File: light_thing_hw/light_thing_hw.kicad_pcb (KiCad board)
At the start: 2 copper layers, 51 parts, among them J1 CONNECTORS, J2 Li-Ion Battery, J3 ADDR_LED_PANEL_1_CONNECTORS, J4 ADDR_LED_PANEL_2_CONNECTORS, Q1 MMBF170, SW1 ST_USER_BUTTON1, SW2 ST_RESET_BUTTON, U1 BC832-V1, U2 LSM6DS3, U3 MCP73833T-FCI_MF, U4 LMR62421XMF, U5 LP38511MRX-ADJ_NOPB, U5A1 STM32L452RETx

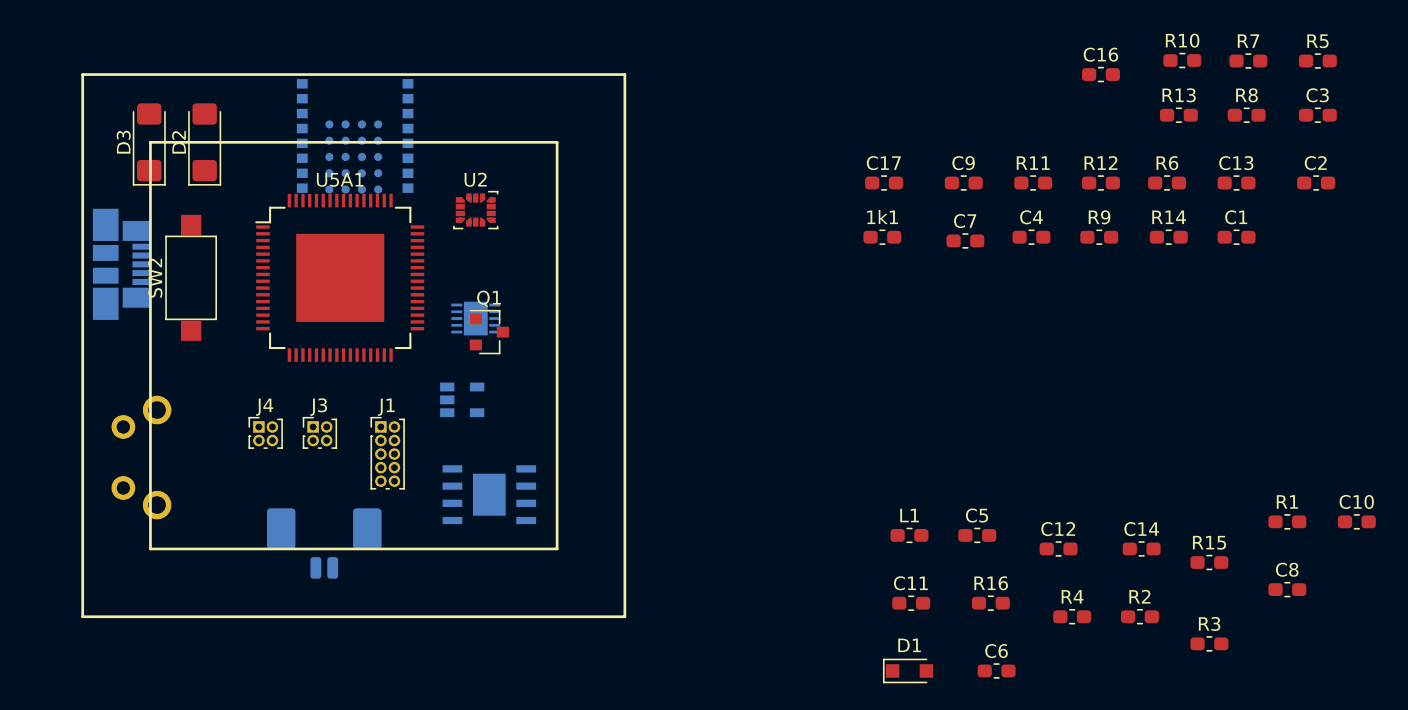
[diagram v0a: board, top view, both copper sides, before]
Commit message: hw updates
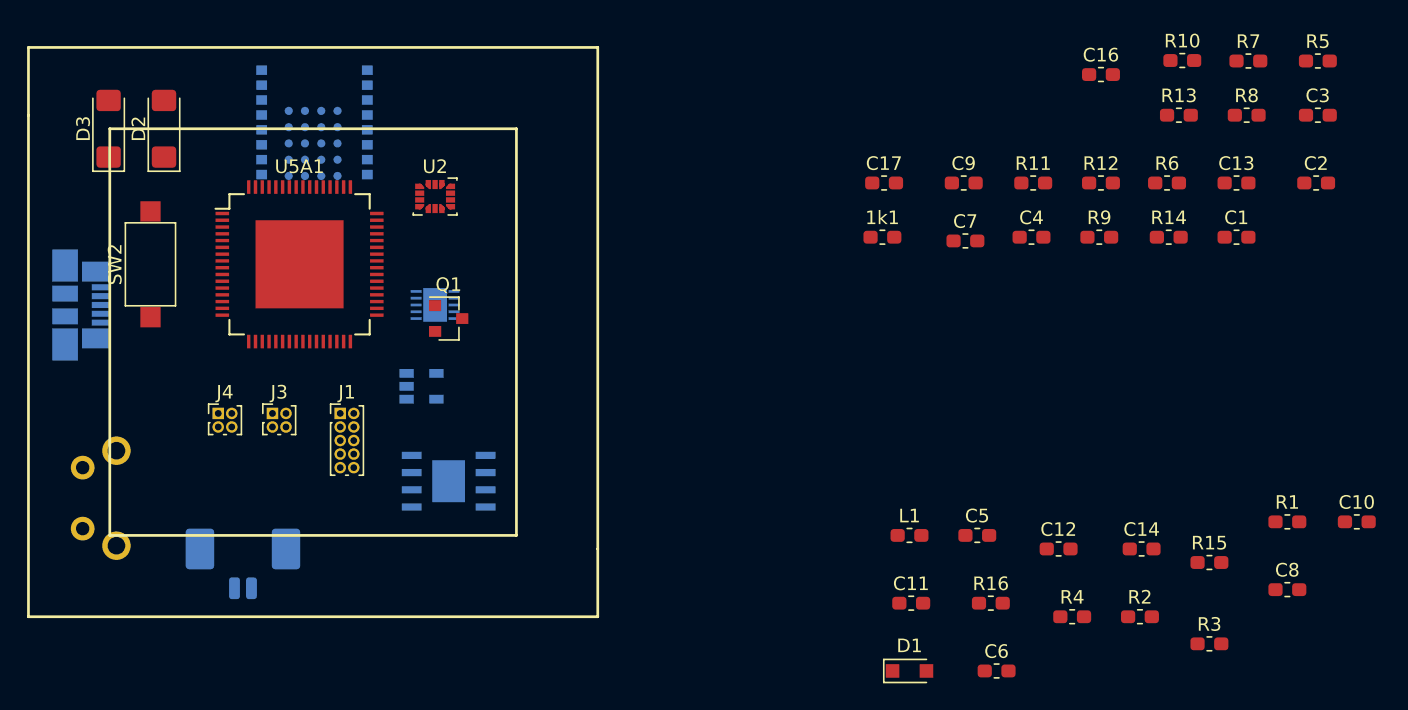
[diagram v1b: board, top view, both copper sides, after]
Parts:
- moved J2 6.18 mm to (166.8, 80.5)
- moved SW1 4.24 mm to (155.0, 74.0)
- moved USB_MICRO_CONN1 4.24 mm to (154.9, 62.0)
- moved D2 3.16 mm to (161.0, 49.0)
- moved D3 3.16 mm to (156.9, 49.0)
- moved J1 3.16 mm to (174.0, 70.0)
- moved J3 3.16 mm to (169.0, 70.0)
- moved J4 3.16 mm to (165.0, 70.0)
- moved Q1 3.16 mm to (182.0, 63.0)
- moved SW2 3.16 mm to (160.0, 59.0)
- moved U1 3.16 mm to (176.0, 53.0)
- moved U2 3.16 mm to (181.0, 54.0)
- moved U3 3.16 mm to (181.0, 62.0)
- moved U4 3.16 mm to (180.0, 68.0)
- moved U5 3.16 mm to (182.0, 75.0)
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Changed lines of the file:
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@@
   (general
     (thickness 1.6)
-    (drawings 11)
+    (drawings 12)
     (tracks 0)
     (zones 0)
@@
   )
   (module LED_SMD:LED_1806_4516Metric_Pad1.57x1.80mm_HandSolder (layer F.Cu)
-    (at 164 50 90)
+    (at 161 49 90)
     (descr "LED SMD 1806 (4516 Metric), square (rectangular) end terminal, IPC_7351 nominal, (Body size source: https://www.modelithics.com/models/Vendor/MuRata/BLM41P.pdf), generated with kicad-footprint-generator")
     (tags "LED handsolder")
@@
   )
   (module LED_SMD:LED_1806_4516Metric_Pad1.57x1.80mm_HandSolder (layer F.Cu)
-    (at 159.9125 50 90)
+    (at 156.9125 49 90)
     (descr "LED SMD 1806 (4516 Metric), square (rectangular) end terminal, IPC_7351 nominal, (Body size source: https://www.modelithics.com/models/Vendor/MuRata/BLM41P.pdf), generated with kicad-footprint-generator")
     (tags "LED handsolder")
@@
   )
   (module Connector_Molex:Molex_PicoBlade_53261-0271_1x02-1MP_P1.25mm_Horizontal (layer B.Cu)
-    (at 172.825 79)
+    (at 166.825 80.5)
     (descr "Molex PicoBlade series connector, 53261-0271 (http://www.molex.com/pdm_docs/sd/532610271_sd.pdf), generated with kicad-footprint-generator")
     (tags "connector Molex PicoBlade top entry")
@@
   )
   (module Connector_PinHeader_1.00mm:PinHeader_2x02_P1.00mm_Vertical (layer F.Cu)
-    (at 172 71)
+    (at 169 70)
     (descr "Through hole straight pin header, 2x02, 1.00mm pitch, double rows")
     (tags "Through hole pin header THT 2x02 1.00mm double row")
@@
   )
   (module Connector_PinHeader_1.00mm:PinHeader_2x02_P1.00mm_Vertical (layer F.Cu)
-    (at 168 71)
+    (at 165 70)
     (descr "Through hole straight pin header, 2x02, 1.00mm pitch, double rows")
     (tags "Through hole pin header THT 2x02 1.00mm double row")
@@
   )
   (module Package_TO_SOT_SMD:SOT-23 (layer F.Cu)
-    (at 185 64)
+    (at 182 63)
     (descr "SOT-23, Standard")
     (tags SOT-23)
@@
   )
   (module Button_Switch_THT:SW_Tactile_SPST_Angled_PTS645Vx39-2LFS (layer B.Cu)
-    (at 158 71 270)
+    (at 155 74 270)
     (descr "tactile switch SPST right angle, PTS645VL39-2 LFS")
     (tags "tactile switch SPST angled PTS645VL39-2 LFS C&K Button")
@@
   )
   (module Button_Switch_SMD:SW_SPST_CK_RS282G05A3 (layer F.Cu)
-    (at 163 60 90)
+    (at 160 59 90)
     (descr https://www.mouser.com/ds/2/60/RS-282G05A-SM_RT-1159762.pdf)
     (tags "SPST button tactile switch")
@@
   )
   (module Package_LGA:LGA-14_3x2.5mm_P0.5mm_LayoutBorder3x4y (layer F.Cu)
-    (at 184 55)
+    (at 181 54)
     (descr "LGA, 14 Pin (http://www.st.com/resource/en/datasheet/lsm6ds3.pdf), generated with kicad-footprint-generator ipc_lga_layoutBorder_generator.py")
     (tags "LGA LGA")
@@
   )
   (module footprints:MCP73833T-FCI&slash_MF (layer B.Cu)
-    (at 184 63)
+    (at 181 62)
     (fp_text reference U3 (at 0 3) (layer B.SilkS)
       (effects (font (size 1 1) (thickness 0.15)) (justify mirror))
@@
   )
   (module Package_TO_SOT_SMD:SOT-23-5 (layer B.Cu)
-    (at 183 69)
+    (at 180 68)
     (descr "5-pin SOT23 package")
     (tags SOT-23-5)
@@
   )
   (module footprints:LP38511MRX-ADJ_NOPB (layer B.Cu)
-    (at 185 76)
+    (at 182 75)
     (fp_text reference U5 (at 0 0) (layer B.SilkS)
       (effects (font (size 1 1) (thickness 0.15)) (justify mirror))
@@
   )
   (module Package_QFP:LQFP-64-1EP_10x10mm_P0.5mm_EP6.5x6.5mm (layer F.Cu)
-    (at 174 60)
+    (at 171 59)
     (descr "64 LEAD LQFP 10x10mm (see MICREL LQFP10x10-64LD-PL-1.pdf and http://www.nxp.com/files/shared/doc/package_info/98ARH98426A.pdf for EP)")
     (tags "QFP 0.5")
@@
   )
   (module Connector_USB:USB_Micro-B_Molex_47346-0001 (layer B.Cu)
-    (at 157.9 59 90)
+    (at 154.9 62 90)
     (descr "Micro USB B receptable with flange, bottom-mount, SMD, right-angle (http://www.molex.com/pdm_docs/sd/473460001_sd.pdf)")
     (tags "Micro B USB SMD")
@@
   )
   (module Connector_PinHeader_1.00mm:PinHeader_2x05_P1.00mm_Vertical (layer F.Cu)
-    (at 177 71)
+    (at 174 70)
     (descr "Through hole straight pin header, 2x05, 1.00mm pitch, double rows")
     (tags "Through hole pin header THT 2x05 1.00mm double row")
@@
   )
   (module Fanstel_modules:BC832-BC832_3d1 (layer B.Cu)
-    (at 179 54 180)
+    (at 176 53 180)
     (attr smd)
     (fp_text reference U1 (at 4.3 9.7 180) (layer B.SilkS)
@@
     )
   )
-  (dimension 30 (width 0.3) (layer F.SilkS)
-    (gr_text "30.000 mm" (at 193.1 65 270) (layer F.SilkS)
+  (gr_line (start 151 48) (end 151 43) (layer F.SilkS) (width 0.2))
+  (gr_line (start 193 80) (end 193 85) (layer F.SilkS) (width 0.2))
+  (dimension 42 (width 0.3) (layer F.SilkS)
+    (gr_text "42.000 mm" (at 140.9 64 90) (layer F.SilkS)
       (effects (font (size 1.5 1.5) (thickness 0.3)))
     )
-    (feature1 (pts (xy 190 80) (xy 191.586421 80)))
-    (feature2 (pts (xy 190 50) (xy 191.586421 50)))
-    (crossbar (pts (xy 191 50) (xy 191 80)))
-    (arrow1a (pts (xy 191 80) (xy 190.413579 78.873496)))
-    (arrow1b (pts (xy 191 80) (xy 191.586421 78.873496)))
-    (arrow2a (pts (xy 191 50) (xy 190.413579 51.126504)))
-    (arrow2b (pts (xy 191 50) (xy 191.586421 51.126504)))
-  )
-  (gr_line (start 190 80) (end 190 50) (layer F.SilkS) (width 0.2))
-  (gr_line (start 160 80) (end 190 80) (layer F.SilkS) (width 0.2))
-  (gr_line (start 160 50) (end 160 80) (layer F.SilkS) (width 0.2))
-  (gr_line (start 190 50) (end 160 50) (layer F.SilkS) (width 0.2))
-  (dimension 40 (width 0.3) (layer F.SilkS)
-    (gr_text "40.000 mm" (at 199.1 65 90) (layer F.SilkS)
+    (feature1 (pts (xy 151 43) (xy 142.413579 43)))
+    (feature2 (pts (xy 151 85) (xy 142.413579 85)))
+    (crossbar (pts (xy 143 85) (xy 143 43)))
+    (arrow1a (pts (xy 143 43) (xy 143.586421 44.126504)))
+    (arrow1b (pts (xy 143 43) (xy 142.413579 44.126504)))
+    (arrow2a (pts (xy 143 85) (xy 143.586421 83.873496)))
+    (arrow2b (pts (xy 143 85) (xy 142.413579 83.873496)))
+  )
+  (gr_line (start 193 43) (end 151 43) (layer F.SilkS) (width 0.2))
+  (gr_line (start 193 80) (end 193 43) (layer F.SilkS) (width 0.2))
+  (gr_line (start 151 85) (end 193 85) (layer F.SilkS) (width 0.2))
+  (gr_line (start 151 48) (end 151 85) (layer F.SilkS) (width 0.2))
+  (dimension 42 (width 0.3) (layer F.SilkS)
+    (gr_text "42.000 mm" (at 172 92.1) (layer F.SilkS)
       (effects (font (size 1.5 1.5) (thickness 0.3)))
     )
-    (feature1 (pts (xy 197 45) (xy 197.586421 45)))
-    (feature2 (pts (xy 197 85) (xy 197.586421 85)))
-    (crossbar (pts (xy 197 85) (xy 197 45)))
-    (arrow1a (pts (xy 197 45) (xy 197.586421 46.126504)))
-    (arrow1b (pts (xy 197 45) (xy 196.413579 46.126504)))
-    (arrow2a (pts (xy 197 85) (xy 197.586421 83.873496)))
-    (arrow2b (pts (xy 197 85) (xy 196.413579 83.873496)))
-  )
-  (dimension 40 (width 0.3) (layer F.SilkS)
-    (gr_text "40.000 mm" (at 175 91.1) (layer F.SilkS)
-      (effects (font (size 1.5 1.5) (thickness 0.3)))
-    )
-    (feature1 (pts (xy 195 89) (xy 195 89.586421)))
-    (feature2 (pts (xy 155 89) (xy 155 89.586421)))
-    (crossbar (pts (xy 155 89) (xy 195 89)))
-    (arrow1a (pts (xy 195 89) (xy 193.873496 89.586421)))
-    (arrow1b (pts (xy 195 89) (xy 193.873496 88.413579)))
-    (arrow2a (pts (xy 155 89) (xy 156.126504 89.586421)))
-    (arrow2b (pts (xy 155 89) (xy 156.126504 88.413579)))
-  )
-  (gr_line (start 195 85) (end 195 45) (layer F.SilkS) (width 0.2))
-  (gr_line (start 155 85) (end 195 85) (layer F.SilkS) (width 0.2))
-  (gr_line (start 155 45) (end 155 85) (layer F.SilkS) (width 0.2))
-  (gr_line (start 195 45) (end 155 45) (layer F.SilkS) (width 0.2))
+    (feature1 (pts (xy 193 85) (xy 193 90.586421)))
+    (feature2 (pts (xy 151 85) (xy 151 90.586421)))
+    (crossbar (pts (xy 151 90) (xy 193 90)))
+    (arrow1a (pts (xy 193 90) (xy 191.873496 90.586421)))
+    (arrow1b (pts (xy 193 90) (xy 191.873496 89.413579)))
+    (arrow2a (pts (xy 151 90) (xy 152.126504 90.586421)))
+    (arrow2b (pts (xy 151 90) (xy 152.126504 89.413579)))
+  )
+  (gr_line (start 187 79) (end 187 49) (layer F.SilkS) (width 0.2))
+  (gr_line (start 157 79) (end 187 79) (layer F.SilkS) (width 0.2))
+  (gr_line (start 157 49) (end 157 79) (layer F.SilkS) (width 0.2))
+  (gr_line (start 187 49) (end 157 49) (layer F.SilkS) (width 0.2))
 )
